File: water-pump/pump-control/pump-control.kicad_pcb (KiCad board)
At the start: 2 copper layers, 18 parts, among them J1 pressure contact, J2 SSR control, J3 Display, J4 Temperature sensors, J5 230V AC, J6 Manual reset, J7 Temperature sensors, SW1 Manual reset, U1 ATmega328P-PU, U2 NRF24L01_Breakout, U3 AMS1117-3.3

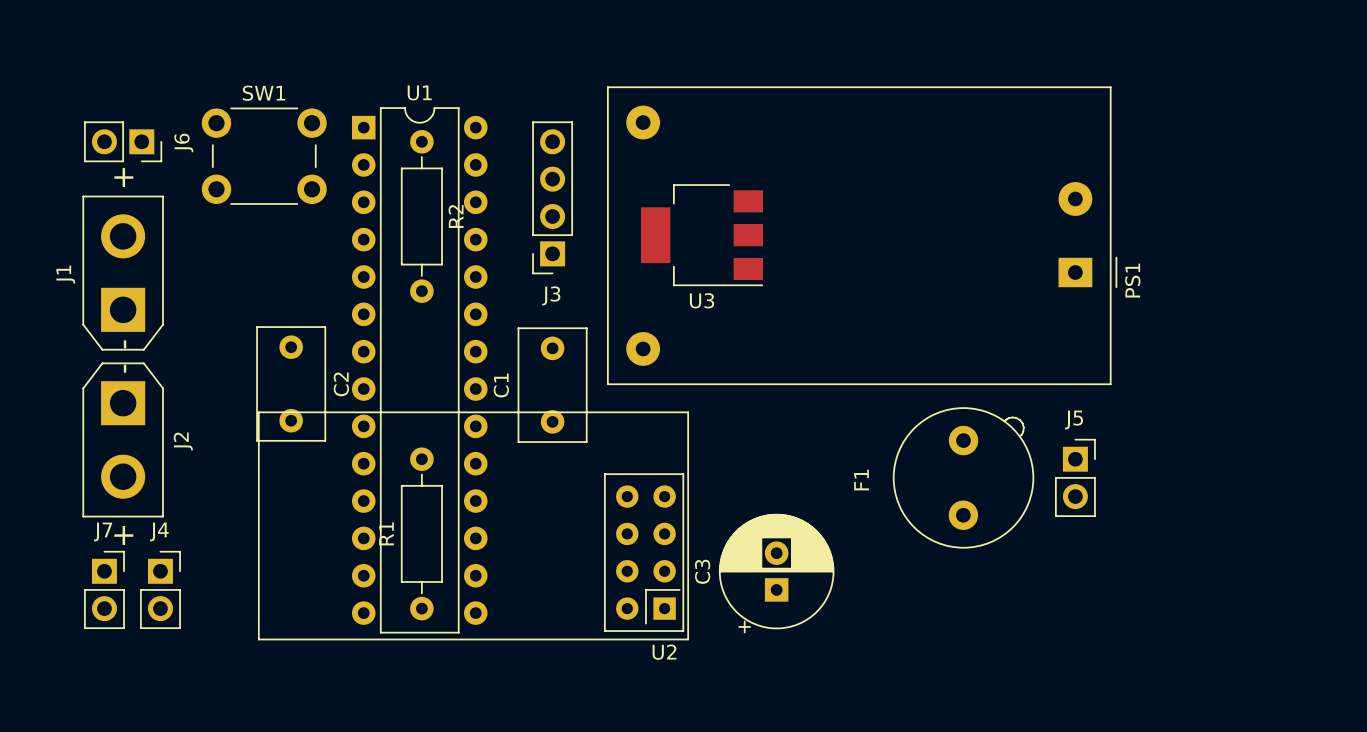
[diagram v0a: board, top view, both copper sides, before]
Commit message: Schema + PCB
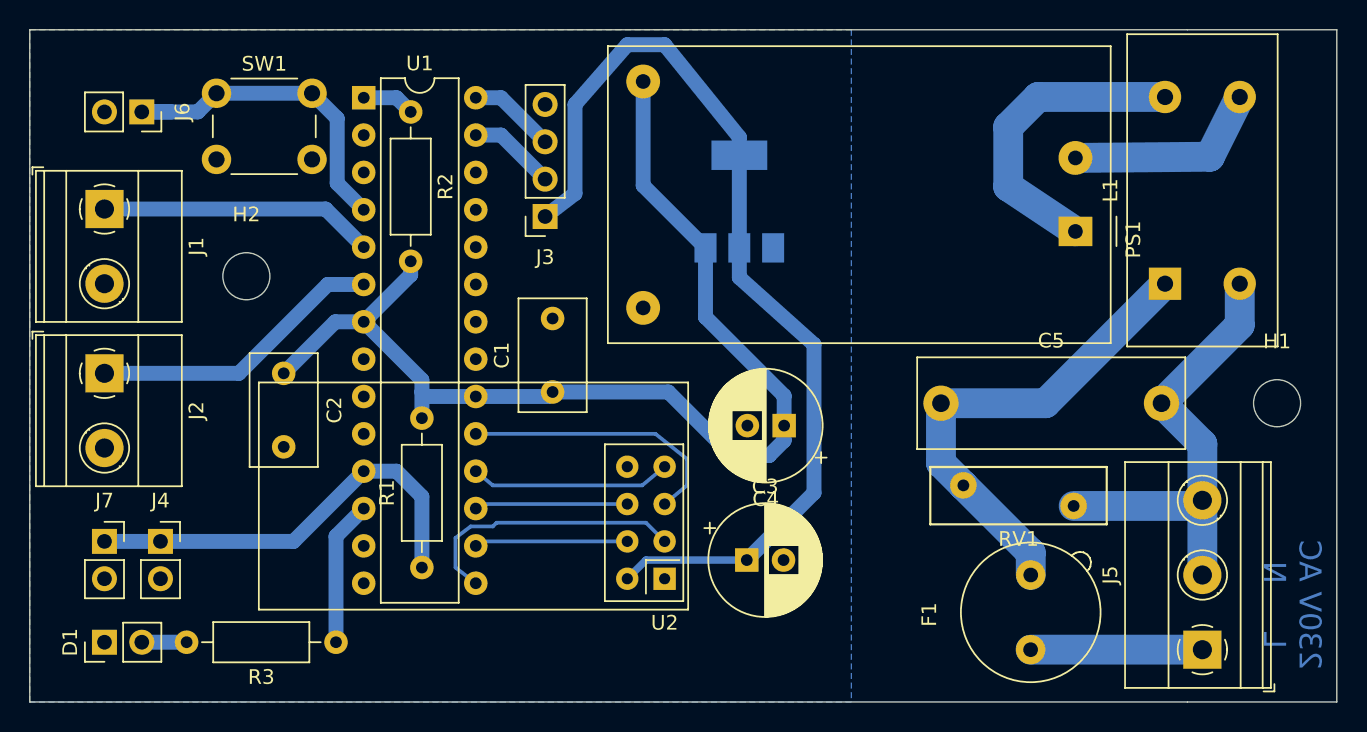
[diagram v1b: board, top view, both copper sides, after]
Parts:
- added C4: 100u, Capacitor_THT:CP_Radial_D7.5mm_P2.50mm, F.Cu at (142.7, 100.6)
- added C5: .1u, Capacitor_THT:C_Rect_L18.0mm_W6.0mm_P15.00mm_FKS3_FKP3, F.Cu at (153.4, 99.1)
- added D1: LED_btn, Connector_PinHeader_2.54mm:PinHeader_1x02_P2.54mm_Vertical, F.Cu at (96.5, 115.3)
- added H1: MountingHole, MountingHole:MountingHole_3.2mm_M3, F.Cu at (176.3, 99.1)
- added H2: MountingHole, MountingHole:MountingHole_3.2mm_M3, F.Cu at (106.2, 90.4)
- added L1: 10mH, Inductor_THT:L_CommonMode_Toroid_Vertical_L21.0mm_W10.0mm_Px5.08mm_Py12.70mm_muRATA_5100, F.Cu at (168.7, 90.9)
- added R3: 330, Resistor_THT:R_Axial_DIN0207_L6.3mm_D2.5mm_P10.16mm_Horizontal, F.Cu at (112.3, 115.3)
- added RV1: 300/450V, Varistor:RV_Disc_D12mm_W3.9mm_P7.5mm, F.Cu at (154.9, 104.6)
- F1: value Fuse_Small -> .5A
- J1, J2: footprint Connector_AMASS:AMASS_XT30UPB-M_1x02_P5.0mm_Vertical -> TerminalBlock_Phoenix:TerminalBlock_Phoenix_MKDS-1,5-2-5.08_1x02_P5.08mm_Horizontal
- J5: footprint Connector_PinSocket_2.54mm:PinSocket_1x02_P2.54mm_Vertical -> TerminalBlock_Phoenix:TerminalBlock_Phoenix_MKDS-1,5-3-5.08_1x03_P5.08mm_Horizontal
- U3: moved to B.Cu
- moved J5 15.6 mm to (171.2, 115.8), turned to 90 degrees
- moved F1 10.2 mm to (159.5, 115.8)
- moved J1 6.97 mm to (96.5, 85.9), turned to 270 degrees
- moved U3 3.42 mm to (139.7, 85.3), turned to 90 degrees
- moved C3 2.87 mm to (140.2, 109.7), turned to 0 degrees
- moved PS1 2.79 mm to (162.6, 87.4)
- moved R1 2.79 mm to (118.1, 110.2)
- moved J3 2.59 mm to (126.5, 86.4)
- moved J2 2.40 mm to (96.5, 97.0)
- moved R2 2.17 mm to (117.3, 79.2)
- moved SW1 2.03 mm to (104.1, 78.0)
- moved C1 2.03 mm to (127.0, 98.3)
- moved J4 2.03 mm to (100.3, 108.5)
- moved J6 2.03 mm to (99.1, 79.2)
- moved J7 2.03 mm to (96.5, 108.5)
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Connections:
- F1 pad 2: Net-(F1-Pad2) -> Net-(C5-Pad1)
- J5 pad 1: Net-(J5-Pad1) -> Net-(F1-Pad1)
- J5 pad 2: Net-(F1-Pad1) -> Net-(C5-Pad2)
- PS1 pad 1: Net-(F1-Pad2) -> Net-(L1-Pad4)
- PS1 pad 2: Net-(J5-Pad1) -> Net-(L1-Pad3)
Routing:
- net +5V: track 0.00 -> 82.4 mm
- net +3V3: track 0.00 -> 66.9 mm
- net Net-(J4-Pad1): track 0.00 -> 42.0 mm
- net Net-(C5-Pad1): track 0.00 -> 32.8 mm
- net Net-(C5-Pad2): track 0.00 -> 32.1 mm
- net Net-(J6-Pad1): track 0.00 -> 23.5 mm
- net Net-(L1-Pad4): track 0.00 -> 21.1 mm
- net Net-(J2-Pad1): track 0.00 -> 20.1 mm
- net /CE: track 0.00 -> 18.9 mm
- net /SCK: track 0.00 -> 18.7 mm
- net Net-(J1-Pad1): track 0.00 -> 18.7 mm
- net Net-(R3-Pad1): track 0.00 -> 16.6 mm
- net Net-(L1-Pad3): track 0.00 -> 13.7 mm
- net /MISO: track 0.00 -> 13.7 mm
- net Net-(F1-Pad1): track 0.00 -> 11.7 mm
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- added copper zone on B.Cu, net GND
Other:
- board outline added: 88.9 x 45.7 mm
- board text added: "230V AC L N"
